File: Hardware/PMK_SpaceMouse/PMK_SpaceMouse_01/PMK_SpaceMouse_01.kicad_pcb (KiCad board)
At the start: 2 copper layers, 60.8 x 61.3 mm, 37 parts, among them J1 FFC2B28-12-G, U1 LDC1614, U2 LDC1612, X1 ASV-40.000MHz

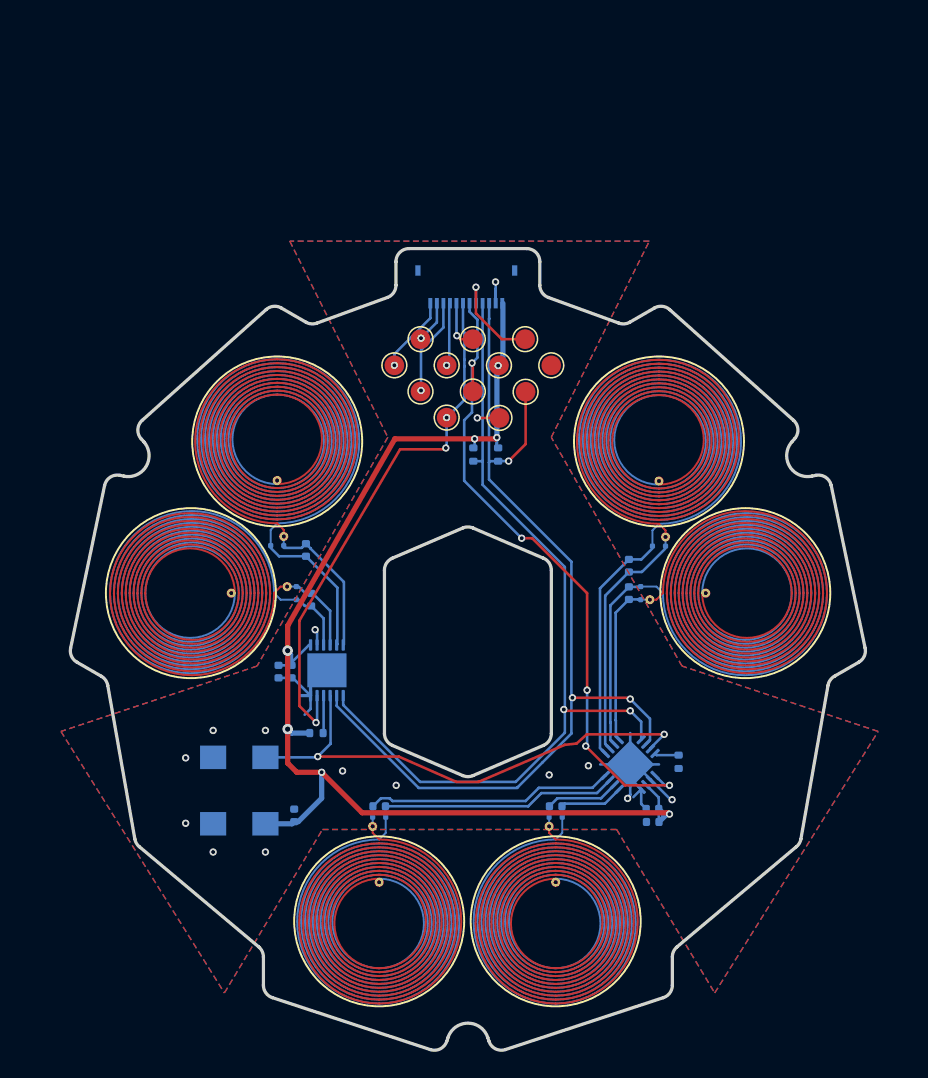
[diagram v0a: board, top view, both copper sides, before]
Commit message: started pmk_03
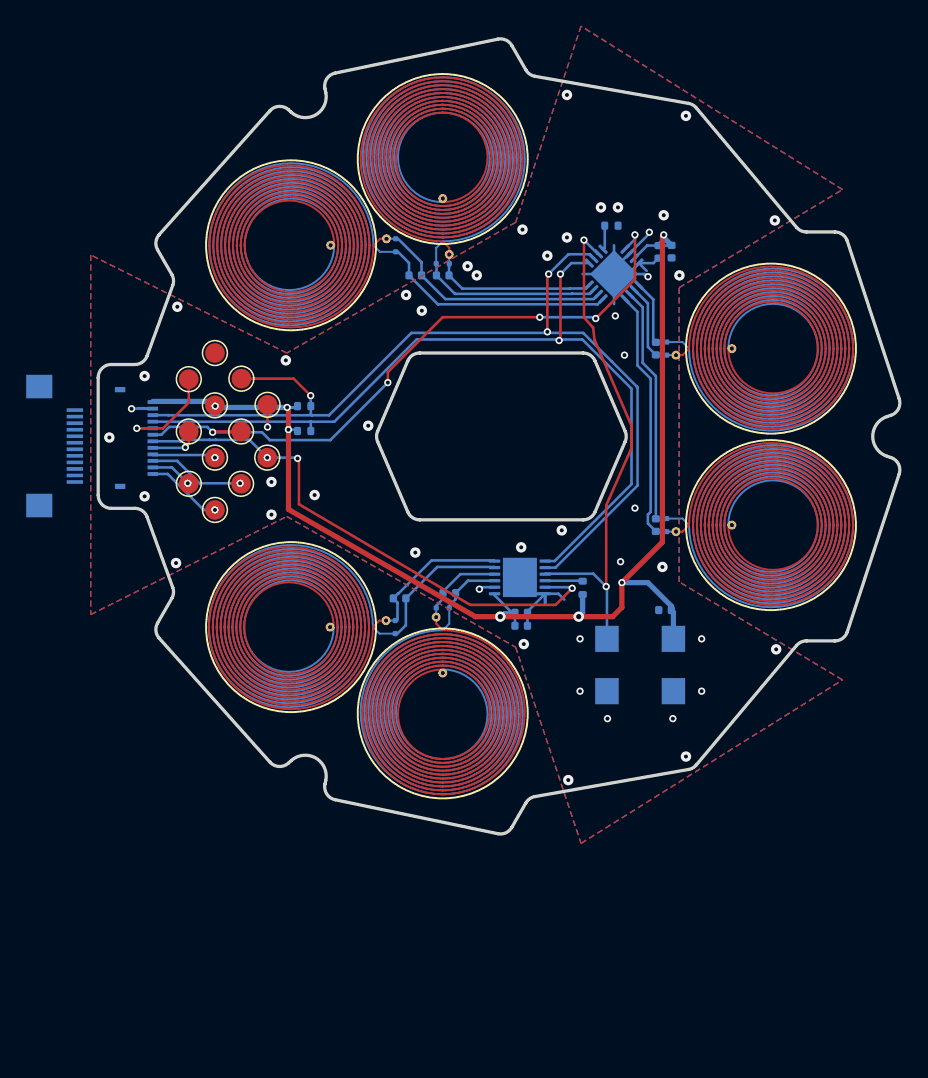
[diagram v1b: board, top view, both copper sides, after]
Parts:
- added J2: vik-module-connector, vik:vik-module-connector-horizontal, B.Cu at (102.7, 86.0)
- moved L1 46.8 mm to (158.2, 79.0), turned to 180 degrees
- moved C9 43.6 mm to (150.4, 71.1), turned to -90 degrees
- moved L2 43.0 mm to (158.2, 92.5), turned to 180 degrees
- moved C8 42.6 mm to (149.4, 71.1), turned to -90 degrees
- moved R1 41.3 mm to (145.8, 69.1), turned to 0 degrees
- moved L4 40.9 mm to (133.4, 63.8), turned to -90 degrees
- moved U1 37.5 mm to (146.0, 72.8), turned to -45 degrees
- moved C1 35.8 mm to (149.2, 78.5), turned to -90 degrees
- moved L3 32.6 mm to (121.1, 70.1), turned to 0 degrees
- moved C12 32.4 mm to (149.9, 98.5), turned to 180 degrees
- moved X1 32.1 mm to (148.0, 102.7), turned to 180 degrees
- moved C2 30.2 mm to (149.2, 92.0), turned to -90 degrees
- moved C4 28.2 mm to (132.9, 72.9), turned to 0 degrees
- moved J1 27.7 mm to (109.4, 85.3), turned to 90 degrees
- moved C3 27.6 mm to (130.8, 72.9), turned to 0 degrees
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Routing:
- net GND: vias 14 -> 46
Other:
- board size 60.8 x 61.3 mm -> 61.3 x 60.8 mm
